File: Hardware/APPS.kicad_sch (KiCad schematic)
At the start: 22 parts, among them SW1 SW_Push, U1 STM32L4P5RET6, Y1 Crystal_GND24

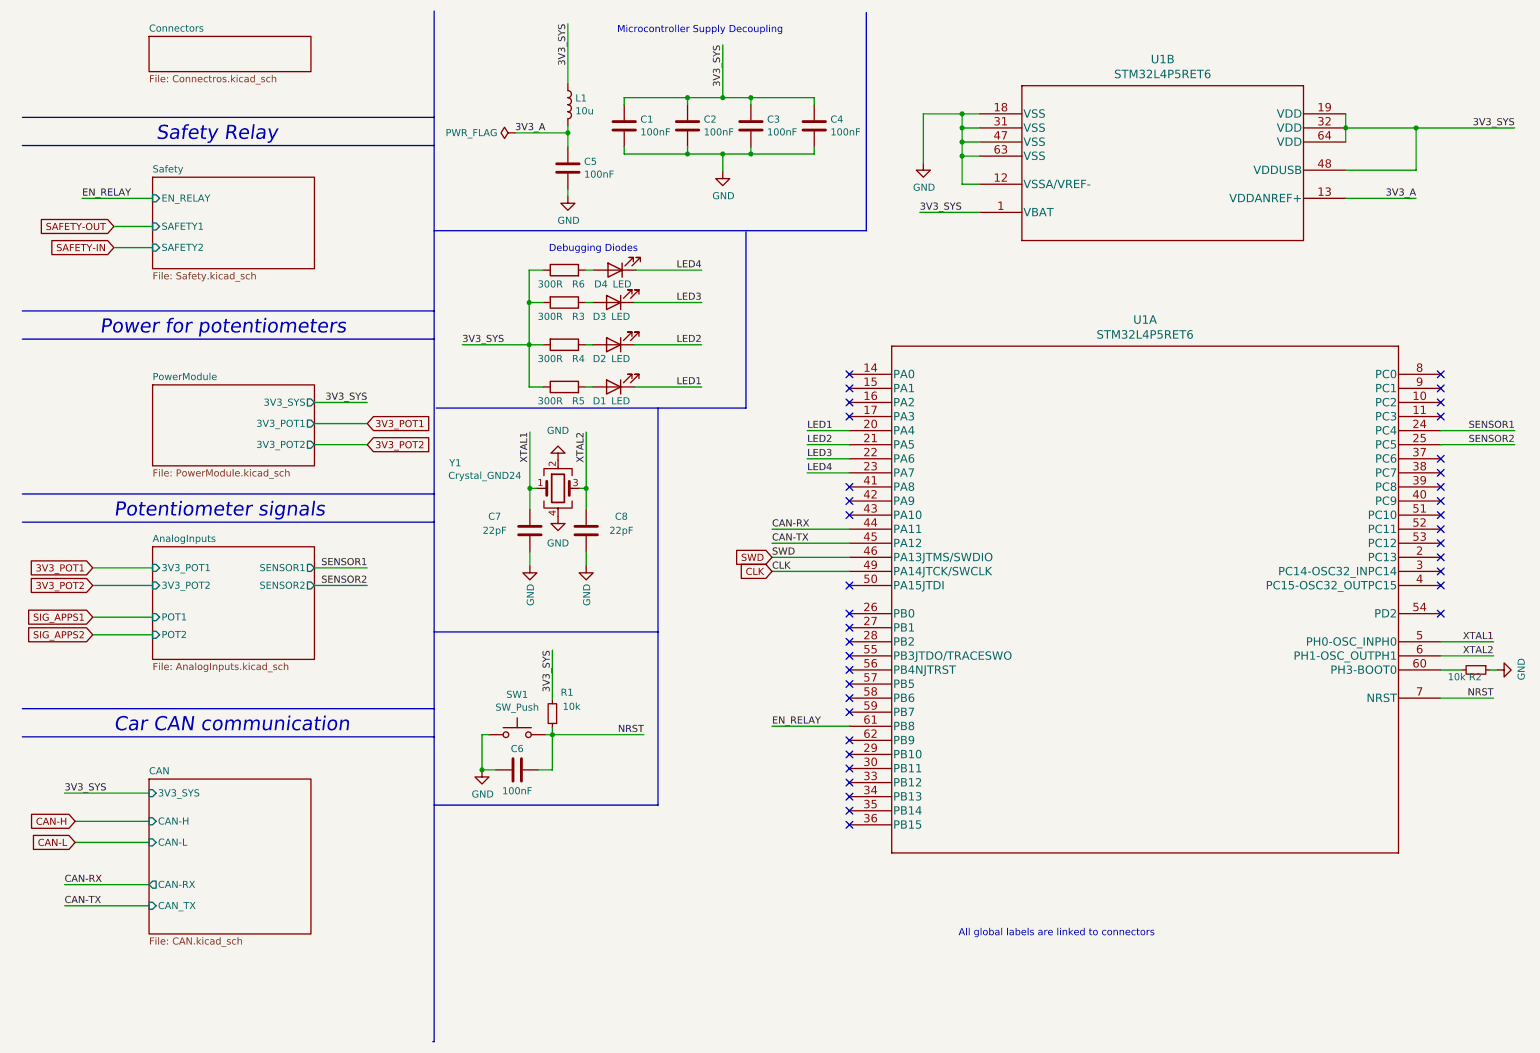
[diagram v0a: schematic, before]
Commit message: Schematic cleanup
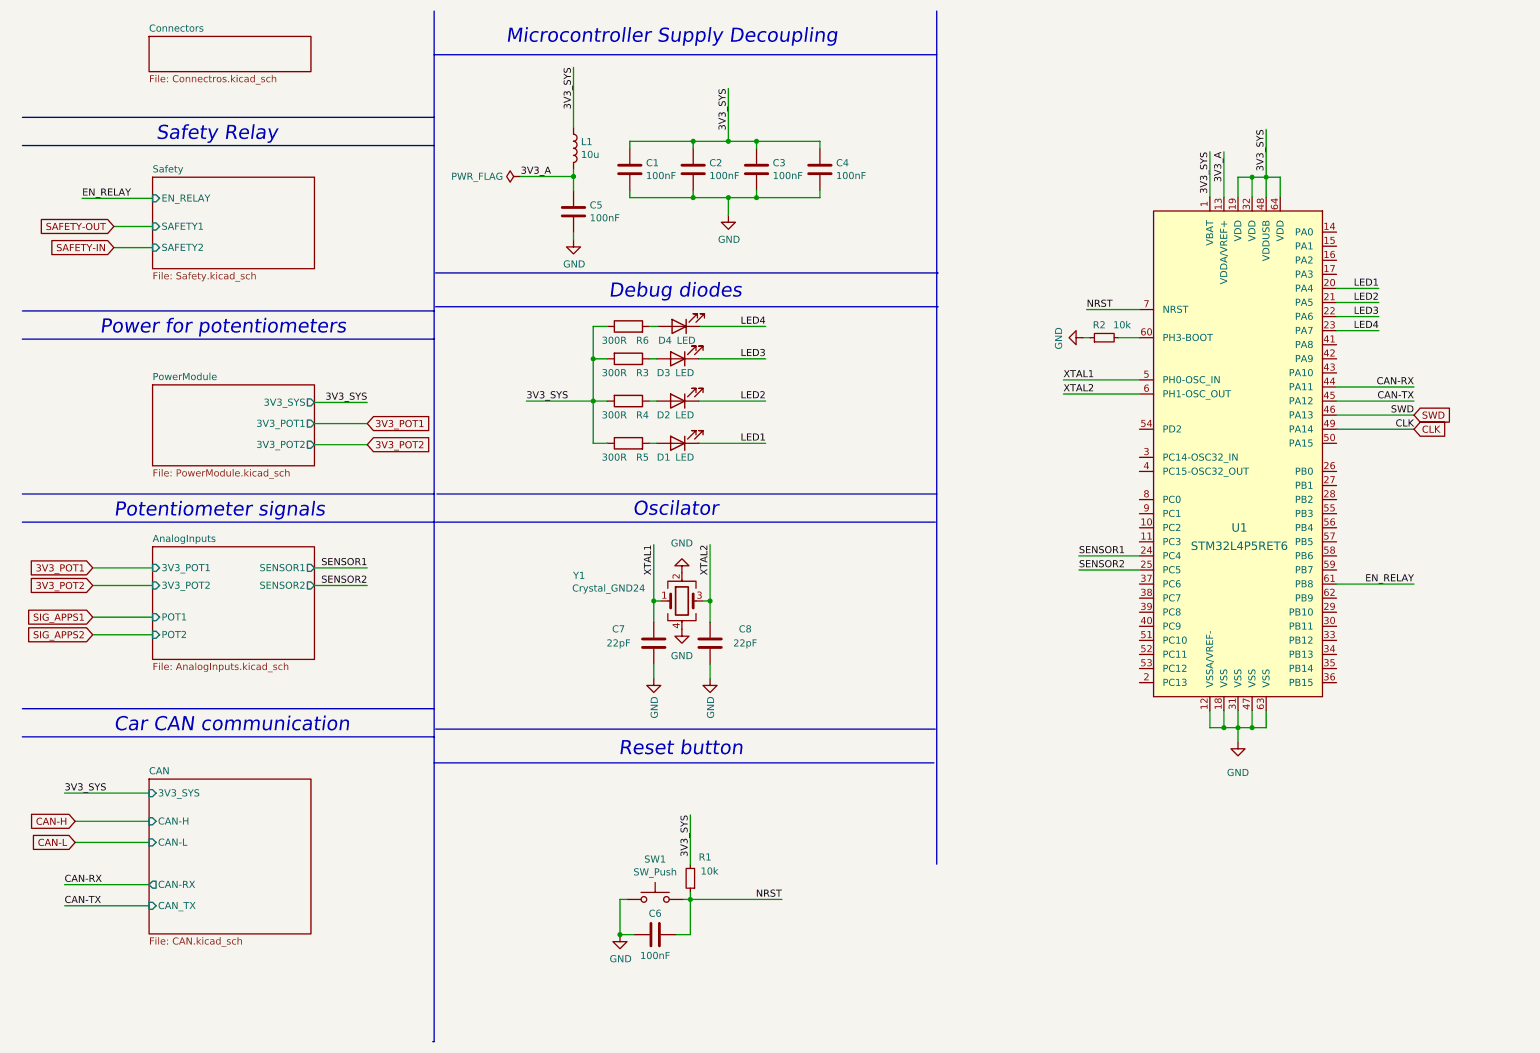
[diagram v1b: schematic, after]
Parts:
- removed unit 2 of U1
- U1: footprint LQFP-64 -> Package_QFP:LQFP-64_10x10mm_P0.5mm; symbol 2021-05-10_08-39-16:STM32L4P5RET6 -> STM32L4P5RET6:STM32L4P5RET6
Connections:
- net 3V3_A: now also U1.13 (VDDA/VREF+)
- net 3V3_SYS: now also U1.1 (VBAT), U1.19 (VDD), U1.32 (VDD), U1.48 (VDDUSB), U1.64 (VDD)
- net GND: now also U1.12 (VSSA/VREF-), U1.18 (VSS), U1.31 (VSS), U1.47 (VSS), U1.63 (VSS)
- no-connect marks 38 -> 0
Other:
- note added: "Debug diodes"
- note added: "Oscilator"
- note added: "Reset button"
- note removed: "All global labels are linked to connectors"
- note removed: "Debugging Diodes"
- title: (none) -> PUT Motorsport EV APPS
- moved on the sheet: C1, C2, C3, C4, C5, C6, C7, C8, D1, D2, D3, D4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
